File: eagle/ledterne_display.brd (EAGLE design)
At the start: 15 x 15 mm, 5 parts

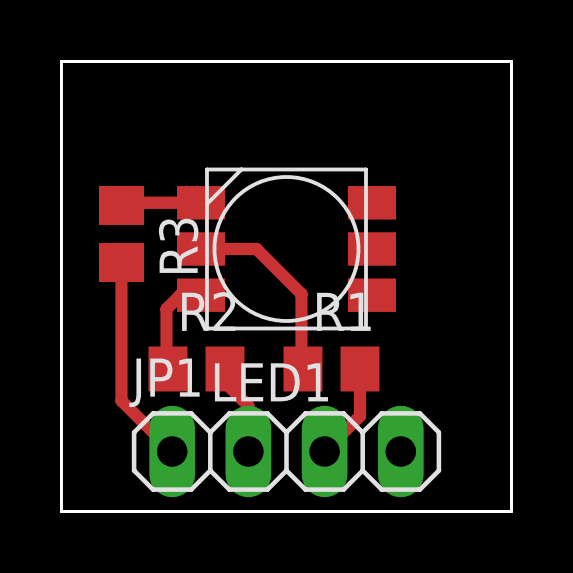
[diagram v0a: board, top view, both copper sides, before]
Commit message: Add ground plane on display board
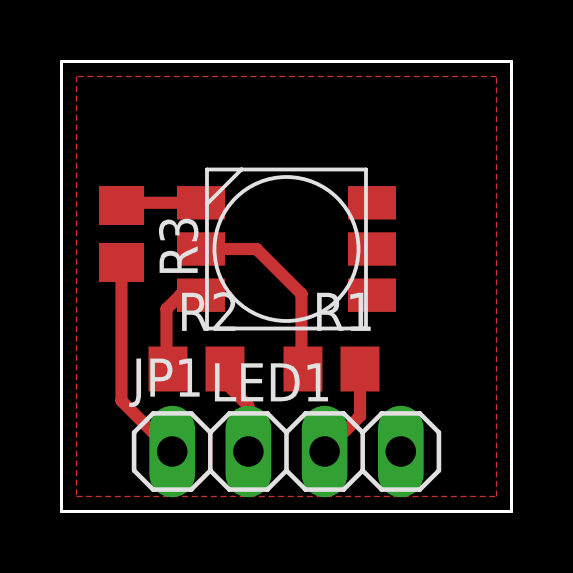
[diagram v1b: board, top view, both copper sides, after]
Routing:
- added copper zone on layer 1, net GND
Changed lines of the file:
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@@
 <contactref element="LED1" pad="P6"/>
 <contactref element="JP1" pad="4"/>
-<wire x1="10.35" y1="8.75" x2="10.35" y2="10.29" width="0" layer="19" extent="1-1"/>
-<wire x1="10.35" y1="7.21" x2="10.35" y2="8.75" width="0" layer="19" extent="1-1"/>
-<wire x1="11.31" y1="2" x2="10.35" y2="7.21" width="0" layer="19" extent="1-1"/>
+<polygon width="0.4" layer="1" isolate="0.4" orphans="yes">
+<vertex x="0.5" y="0.5"/>
+<vertex x="14.5" y="0.5"/>
+<vertex x="14.5" y="14.5"/>
+<vertex x="0.5" y="14.5"/>
+</polygon>
 </signal>
 <signal name="LED_R">
